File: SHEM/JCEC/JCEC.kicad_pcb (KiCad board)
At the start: 2 copper layers, 41 parts, among them U1 TL082, U2 TL082, U3 TL082, U4 TL082, U5 TL082

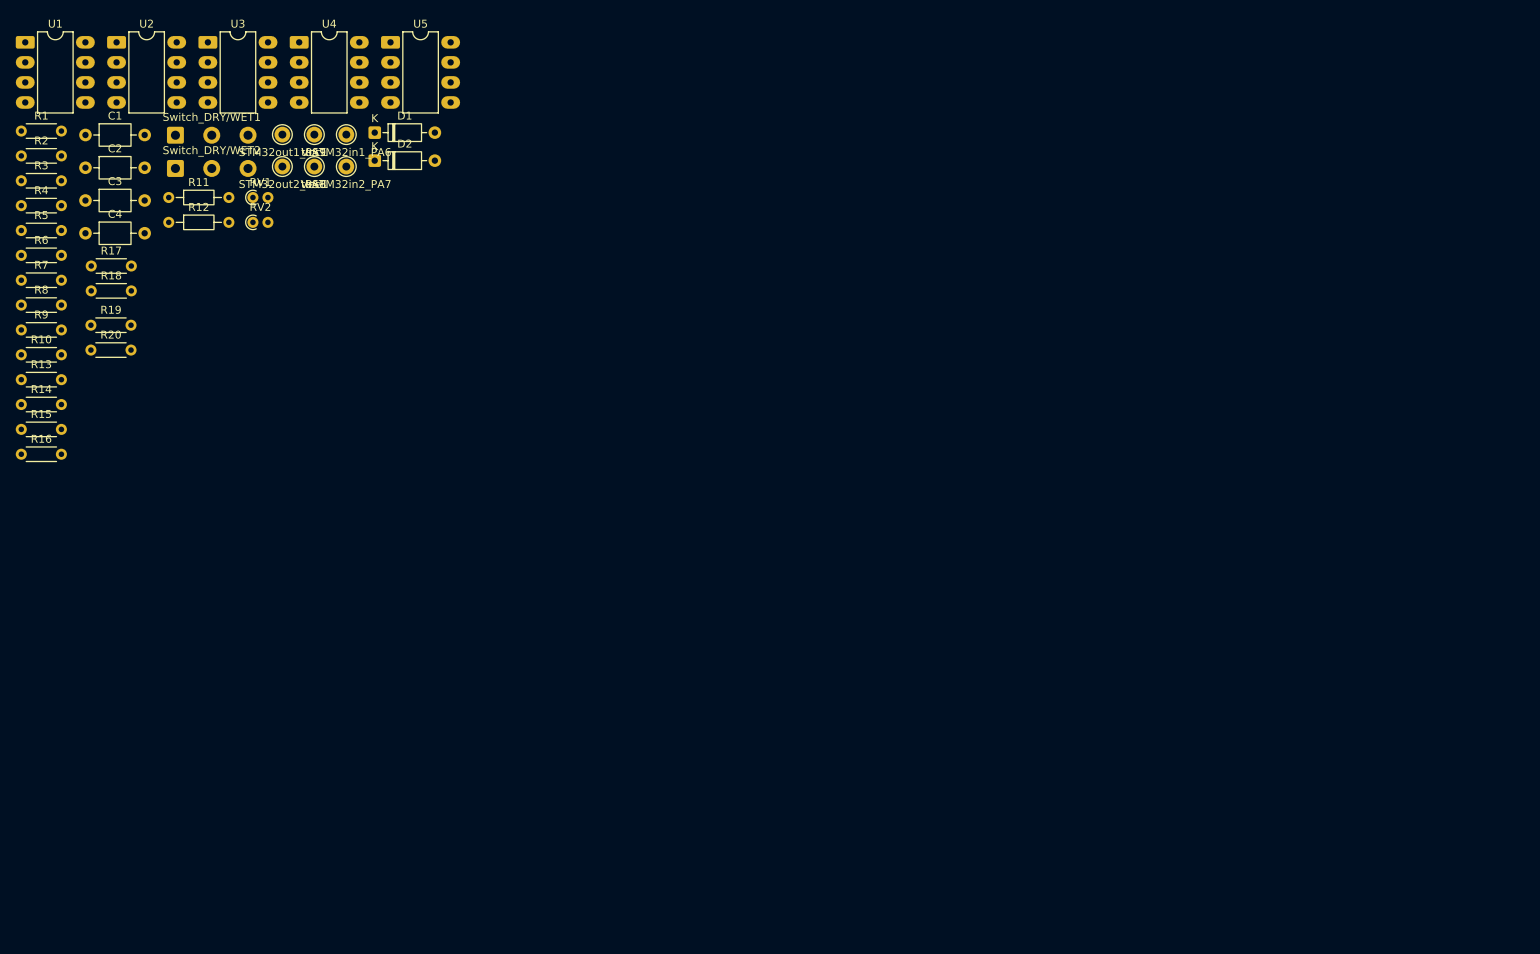
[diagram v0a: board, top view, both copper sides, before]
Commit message: Update
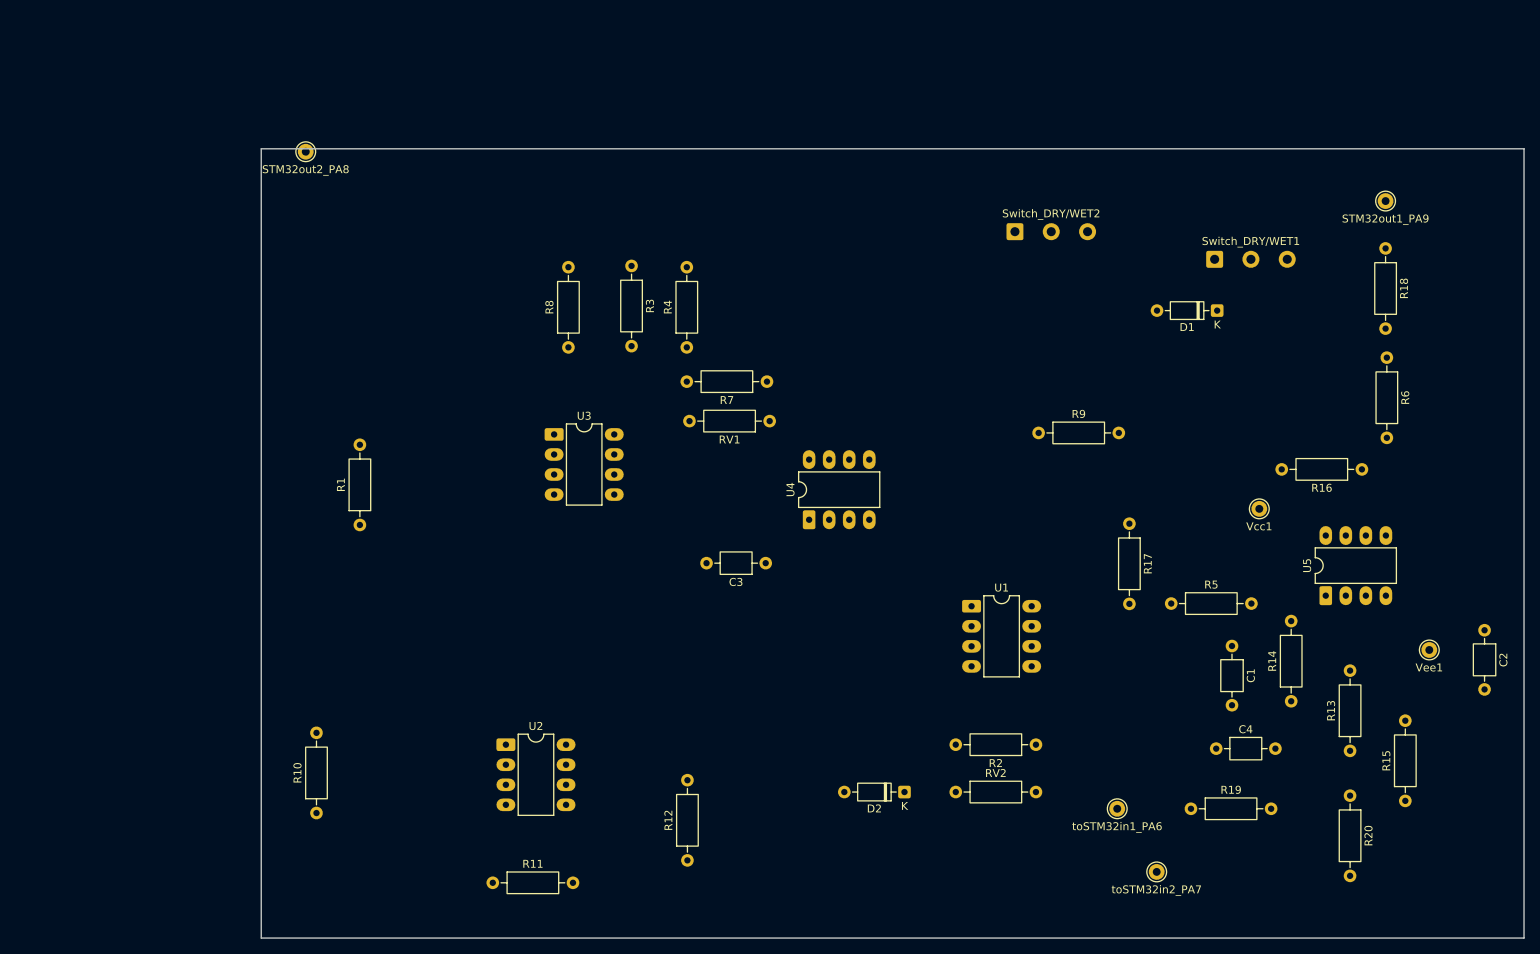
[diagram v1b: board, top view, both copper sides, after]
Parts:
- C3: value 1µ / 2,2µ / 10µ -> 10µ
- R1, R10, R13, R14, R15, R16, R17, R18, R19, R2, R20, R3, R4, R5, R6, R7, R8, R9: footprint Resistor_THT:R_Axial_DIN0204_L3.6mm_D1.6mm_P5.08mm_Horizontal -> Resistor_THT:R_Axial_DIN0207_L6.3mm_D2.5mm_P10.16mm_Horizontal
- R11, R12: footprint Resistor_THT:R_Axial_DIN0204_L3.6mm_D1.6mm_P7.62mm_Horizontal -> Resistor_THT:R_Axial_DIN0207_L6.3mm_D2.5mm_P10.16mm_Horizontal
- RV1, RV2: footprint Resistor_THT:R_Axial_DIN0204_L3.6mm_D1.6mm_P1.90mm_Vertical -> Resistor_THT:R_Axial_DIN0207_L6.3mm_D2.5mm_P10.16mm_Horizontal
- moved C2 186.7 mm to (202.5, 94.0), turned to -90 degrees
- moved R15 181.6 mm to (192.5, 115.6), turned to 90 degrees
- moved R13 174.8 mm to (185.5, 109.3), turned to 90 degrees
- moved R6 173.5 mm to (190.1, 59.5), turned to -90 degrees
- moved R16 169.9 mm to (187.0, 73.6), turned to 180 degrees
- moved R20 169.2 mm to (185.5, 115.0), turned to -90 degrees
- moved R14 165.2 mm to (178.0, 103.0), turned to 90 degrees
- moved R18 164.1 mm to (190.0, 45.6), turned to -90 degrees
- moved C1 159.0 mm to (170.5, 96.0), turned to -90 degrees
- moved C4 157.4 mm to (168.5, 109.0)
- moved Vee1 154.0 mm to (195.5, 96.5)
- moved R5 153.2 mm to (162.8, 90.6)
- moved R19 152.3 mm to (165.3, 116.6)
- moved R2 148.6 mm to (145.7, 108.5), turned to 180 degrees
- moved STM32out1_PA9 140.0 mm to (190.0, 39.6)
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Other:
- board outline added: 160 x 100 mm
